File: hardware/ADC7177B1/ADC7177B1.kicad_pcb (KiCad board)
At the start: 2 copper layers, 55 parts, among them J1 20021111-00010T4LF, J2 RJ45_Wuerth_7499010121A, U1 STM32H743VITx, U2 24LC08B-E/MS, U3 LAN8742A, U5 TPS7A4901DGN, U6 ADC7177M1, U7 TPS7A3001DGN

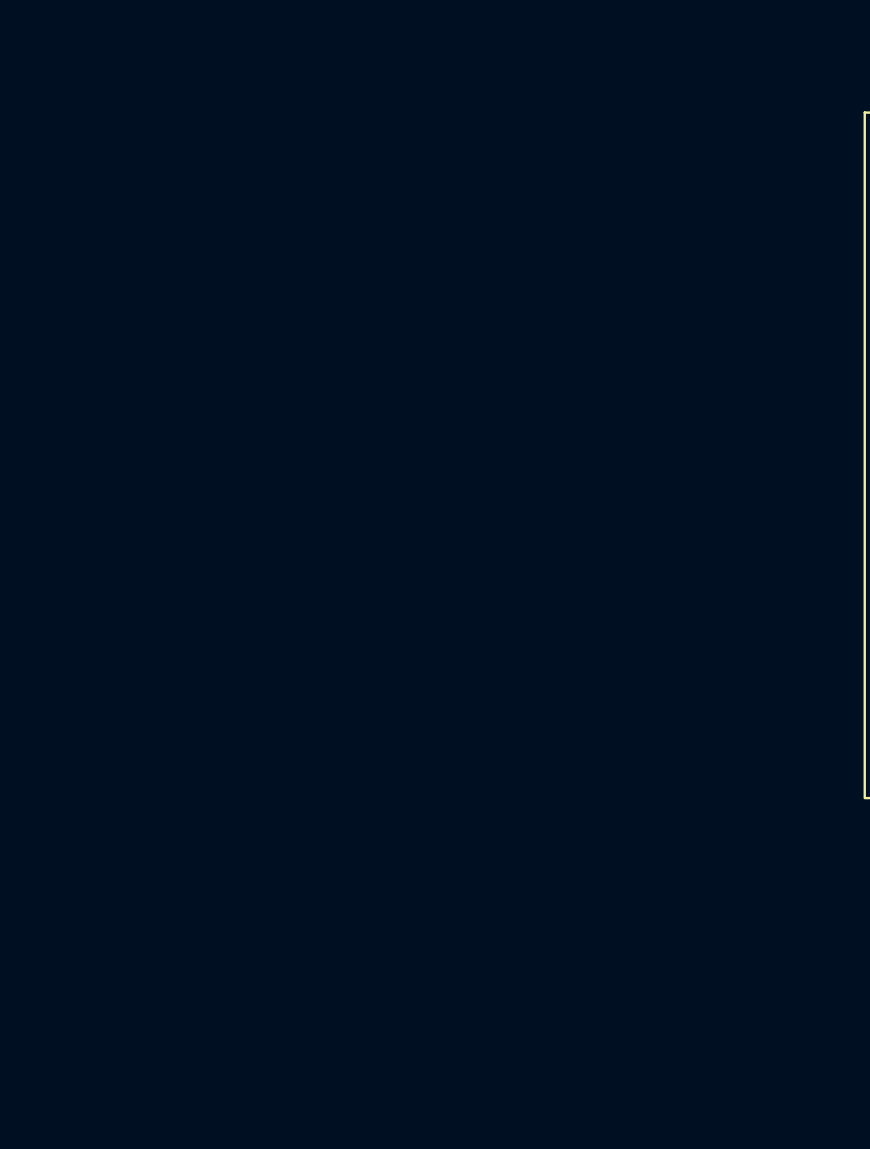
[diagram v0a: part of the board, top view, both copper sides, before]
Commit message: Schematic and PCB
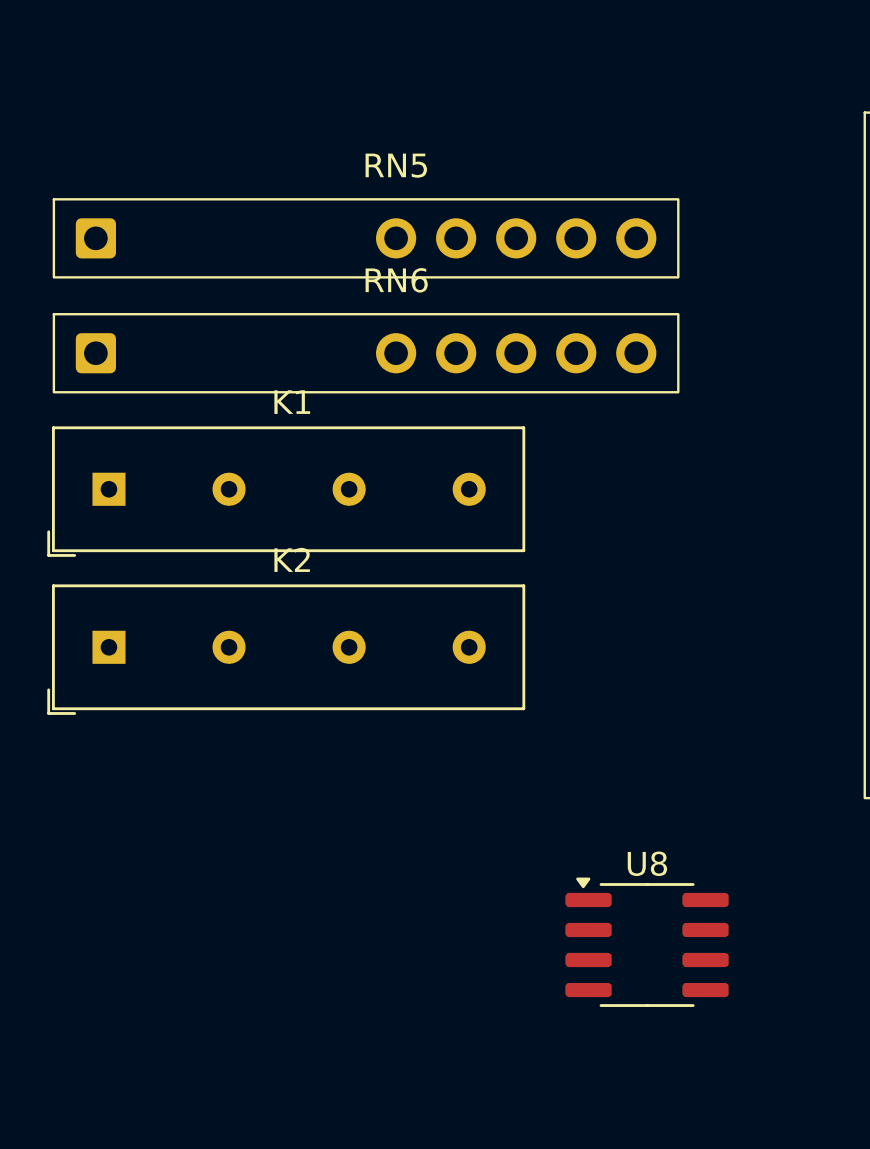
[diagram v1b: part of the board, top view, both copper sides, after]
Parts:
- added K1: SILxx-1Axx-71x, Relay_THT:Relay_SPST_StandexMeder_SIL_Form1A, F.Cu at (91.8, 76.3)
- added K2: SILxx-1Axx-71x, Relay_THT:Relay_SPST_StandexMeder_SIL_Form1A, F.Cu at (91.8, 83.0)
- added RN5: 1776-C68xx, ADC7177B1:1776-C68xx, F.Cu at (103.9, 65.7)
- added RN6: 1776-C68xx, ADC7177B1:1776-C68xx, F.Cu at (103.9, 70.6)
- added U8: AD8599ARZ, Package_SO:SOIC-8_3.9x4.9mm_P1.27mm, F.Cu at (114.5, 95.6)
